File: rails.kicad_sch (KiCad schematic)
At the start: 85 parts, among them U13 LM61460AASQRJRRQ1, U5 TPS259474ARPWR, U6 LM61460AASQRJRRQ1

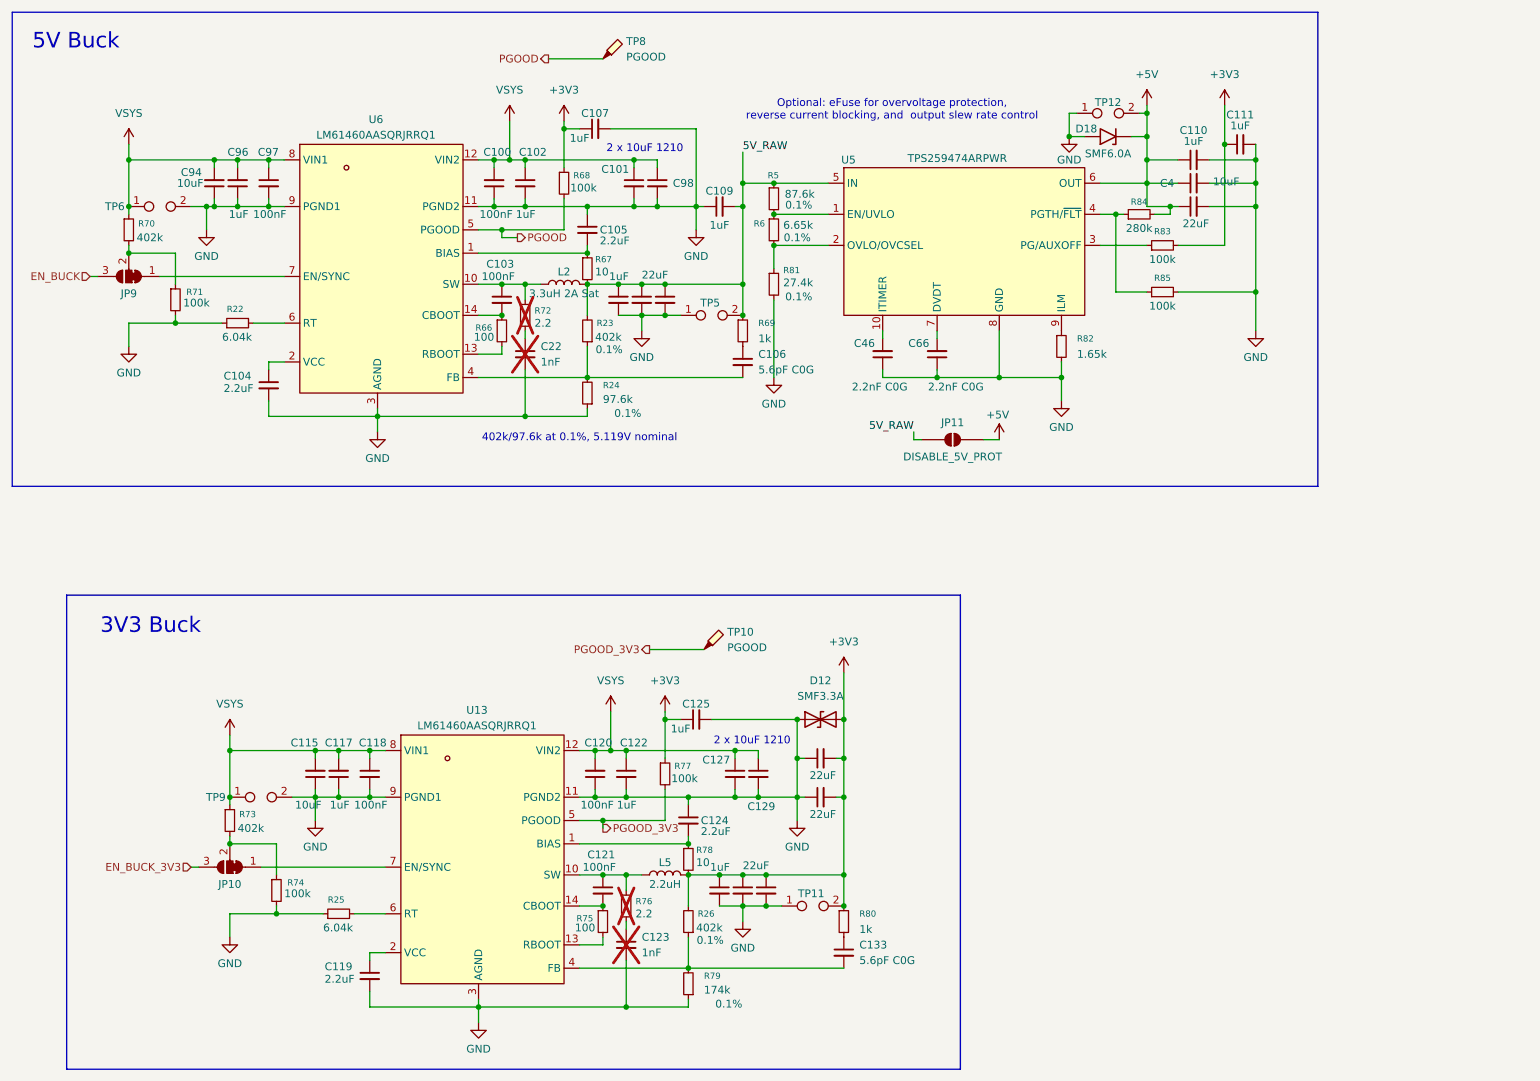
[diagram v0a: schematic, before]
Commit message: usb-org
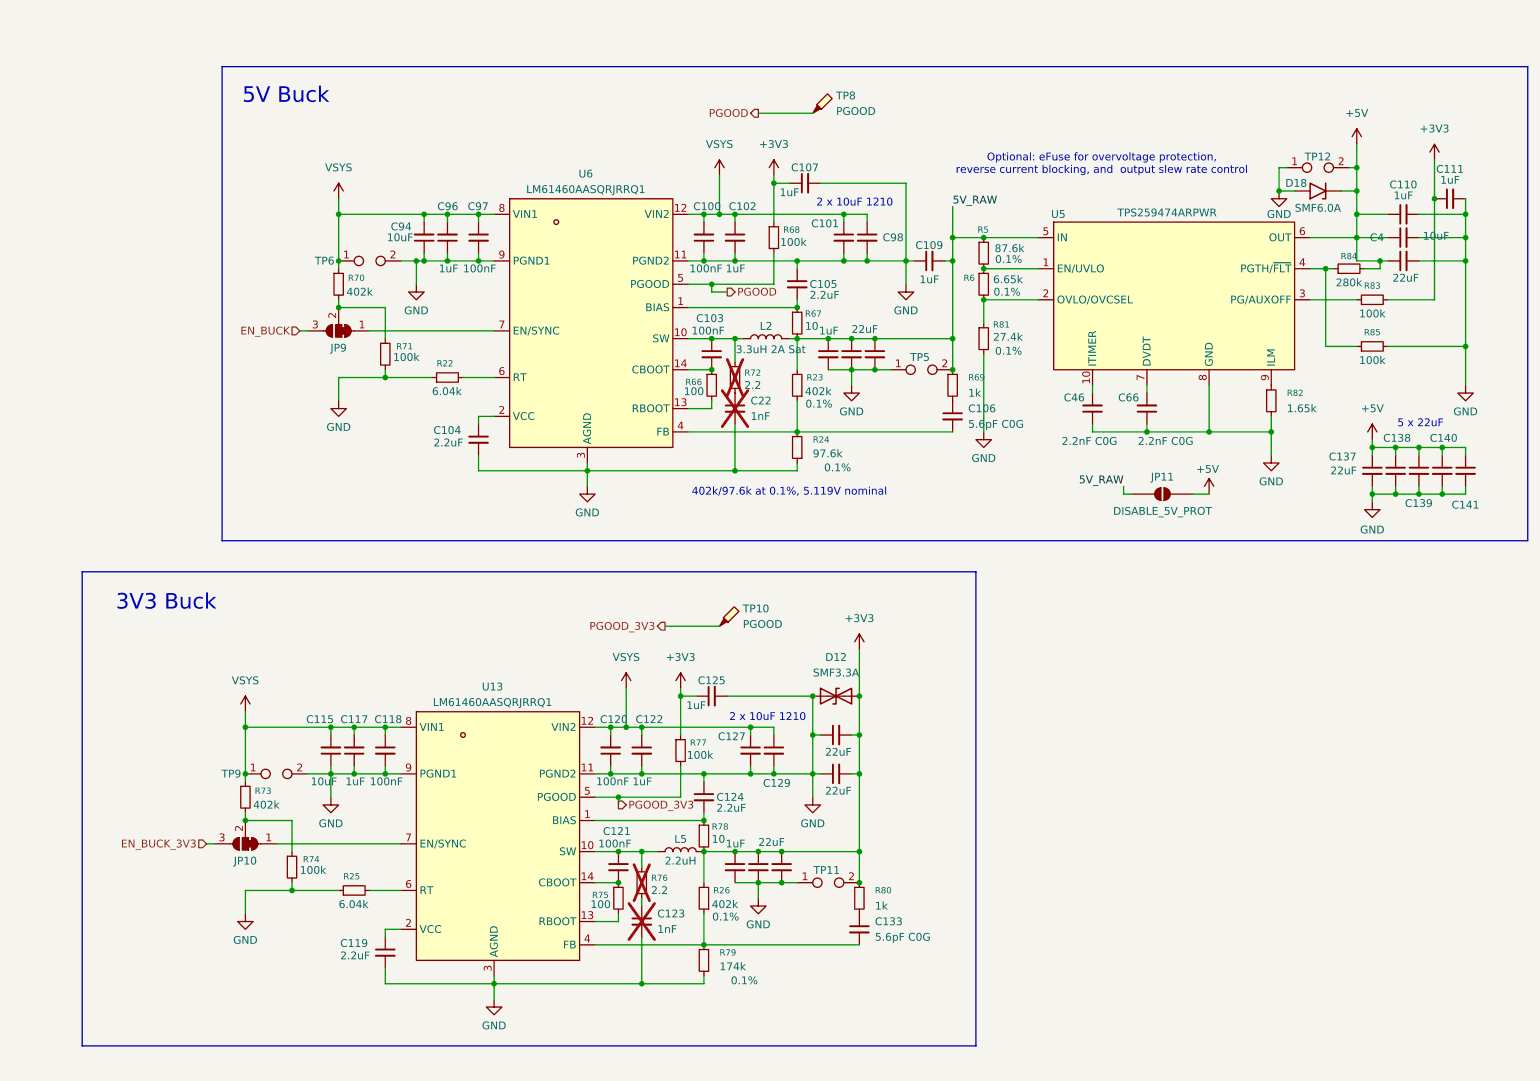
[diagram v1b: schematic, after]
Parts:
- added C137, C138, C139, C140, C141: 22uF, Capacitor_SMD:C_1210_3225Metric, symbol Device:C_Small
- L2: LCSC Part C3002593 -> (none)
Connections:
- net +5V: now also C137.1, C138.1, C139.1, C140.1, C141.1
- net GND: now also C137.2, C138.2, C139.2, C140.2, C141.2
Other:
- note added: "5 x 22uF"
- moved on the sheet: C100, C101, C102, C103, C104, C105, C106, C107, C109, C110, C111, C115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
